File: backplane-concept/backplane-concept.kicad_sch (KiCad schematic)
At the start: 77 parts, among them IC1 ISO6760DWR, IC2 ISO6760DWR, J1 ECVT I/O, J11 1-967657-1, J12 POWER, J2 PCIE_8x_Labeled, J3 PCIE_8x_Labeled, J4 PCIE_8x_Labeled, J5 CONN_MINI, J6 CONN_MINI, J7 CONN_MINI, J8 CONN_MINI

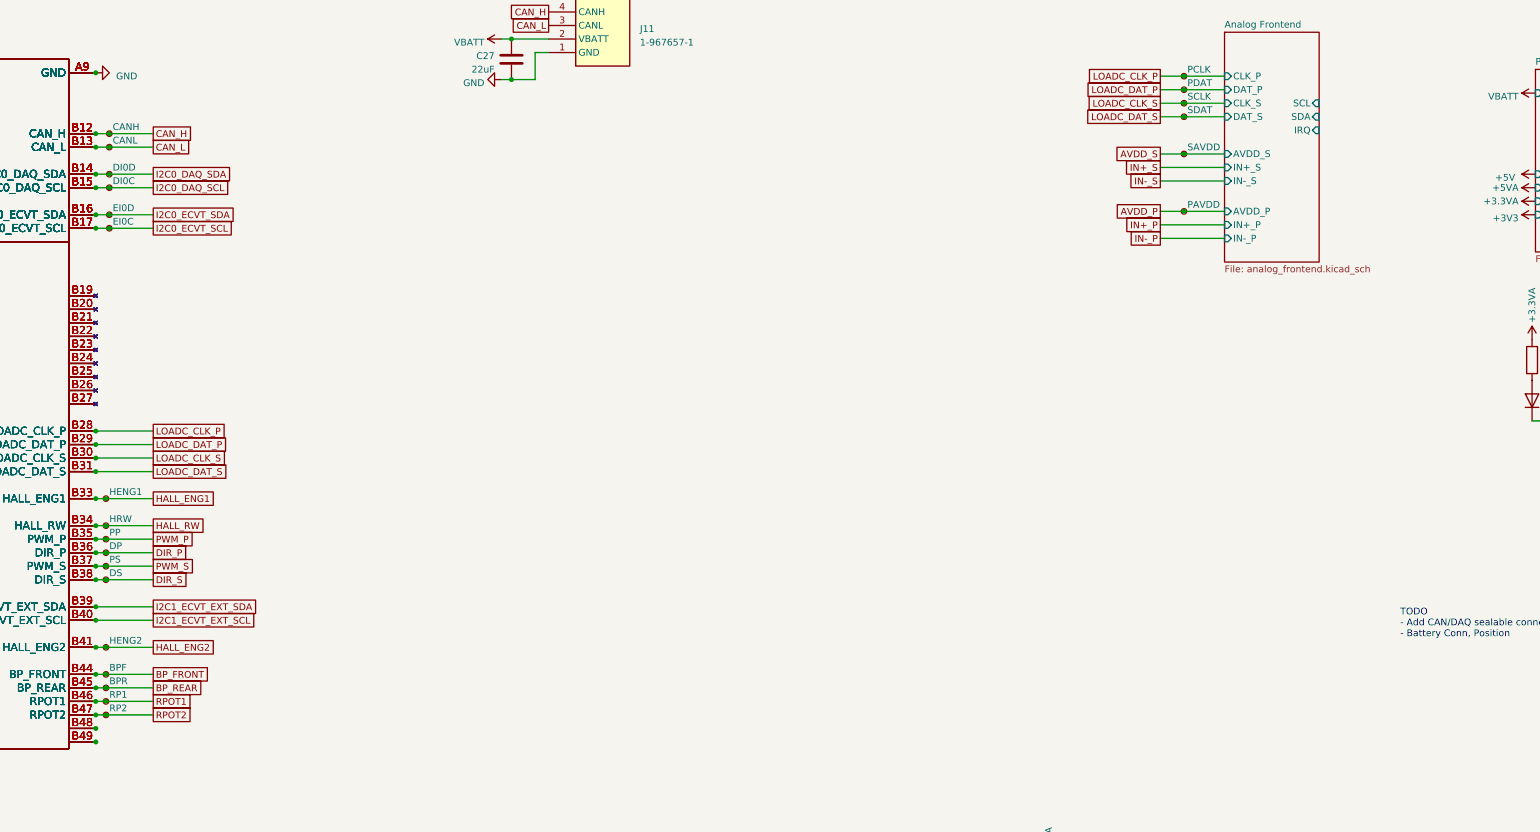
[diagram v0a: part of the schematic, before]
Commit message: Finish Routing
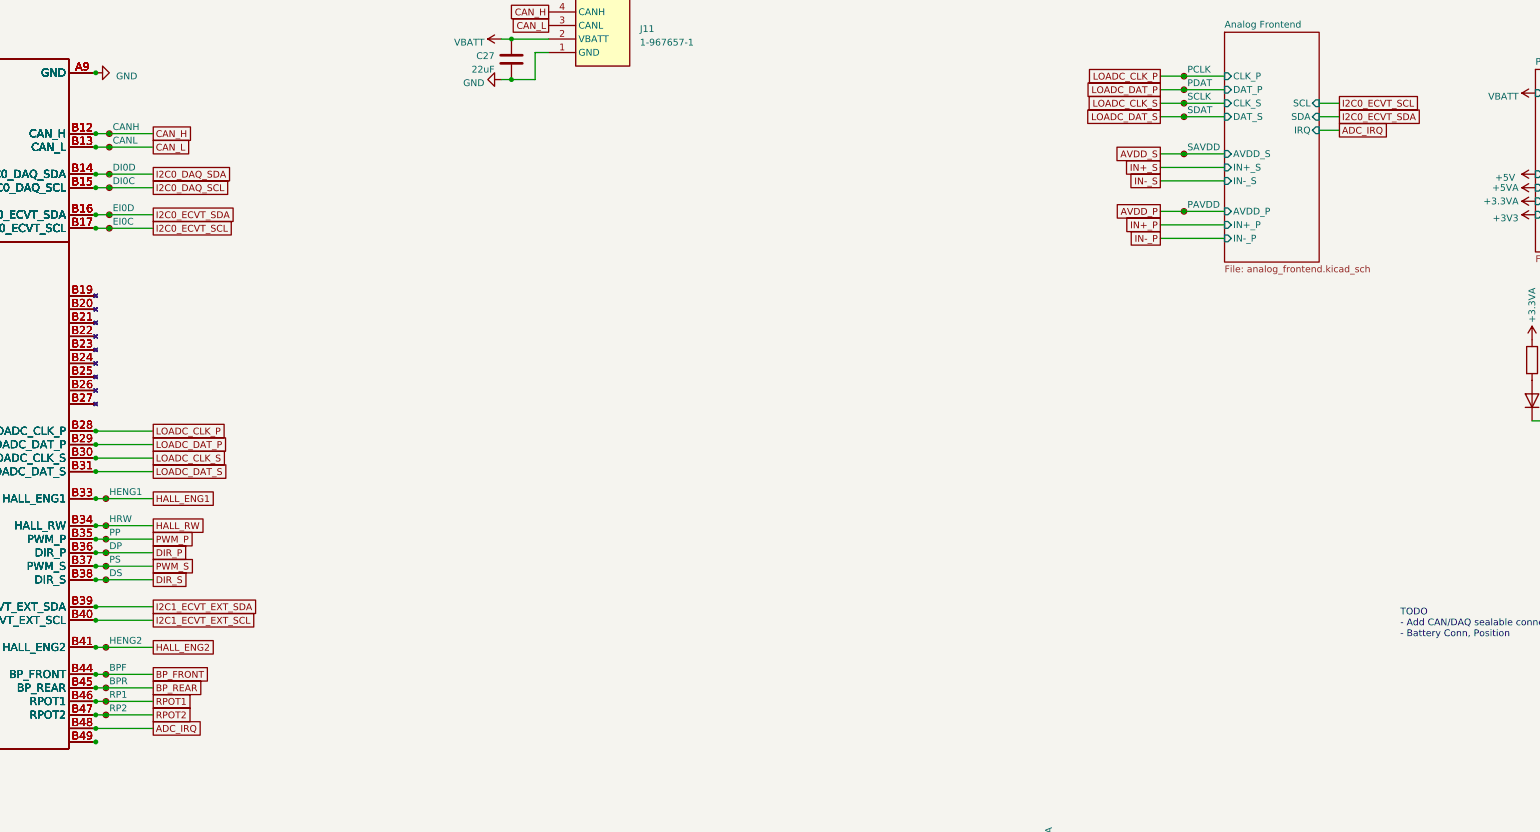
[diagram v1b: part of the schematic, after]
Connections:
- net ADC_IRQ: now reaches J2.B48, J3.B48, J4.B48
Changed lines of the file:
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@@
+    (stroke (width 0) (type default))
+  )
+  (wire (pts (xy 326.39 34.29) (xy 330.2 34.29))
     (stroke (width 0) (type default))
   )
@@
     (stroke (width 0) (type default))
   )
+  (wire (pts (xy 96.52 149.225) (xy 107.315 149.225))
+    (stroke (width 0) (type default))
+  )
   (wire (pts (xy 107.315 100.965) (xy 96.52 100.965))
     (stroke (width 0) (type default))
@@
     (stroke (width 0) (type default))
   )
+  (wire (pts (xy 326.39 36.83) (xy 330.2 36.83))
+    (stroke (width 0) (type default))
+  )
   (wire (pts (xy 36.195 121.285) (xy 38.1 121.285))
     (stroke (width 0) (type default))
@@
   )
   (wire (pts (xy 107.315 113.665) (xy 98.425 113.665))
+    (stroke (width 0) (type default))
+  )
+  (wire (pts (xy 326.39 31.75) (xy 330.2 31.75))
     (stroke (width 0) (type default))
   )
@@
     )
   )
+  (global_label "ADC_IRQ" (shape passive) (at 330.2 36.83 0) (fields_autoplaced)
+    (effects (font (size 1.27 1.27)) (justify left))
+    (property "Intersheetrefs" "${INTERSHEET_REFS}" (at 339.796 36.83 0)
+      (effects (font (size 1.27 1.27)) (justify left) hide)
+    )
+  )
   (global_label "I2C0_ECVT_SDA" (shape passive) (at 107.315 52.705 0) (fields_autoplaced)
     (effects (font (size 1.27 1.27)) (justify left))
@@
     (property "Intersheetrefs" "${INTERSHEET_REFS}" (at 289.0052 57.15 0)
       (effects (font (size 1.27 1.27)) (justify right) hide)
+    )
+  )
+  (global_label "I2C0_ECVT_SCL" (shape passive) (at 330.2 31.75 0) (fields_autoplaced)
+    (effects (font (size 1.27 1.27)) (justify left))
+    (property "Intersheetrefs" "${INTERSHEET_REFS}" (at 346.2063 31.75 0)
+      (effects (font (size 1.27 1.27)) (justify left) hide)
     )
   )
@@
     )
   )
+  (global_label "ADC_IRQ" (shape passive) (at 107.315 149.225 0) (fields_autoplaced)
+    (effects (font (size 1.27 1.27)) (justify left))
+    (property "Intersheetrefs" "${INTERSHEET_REFS}" (at 116.911 149.225 0)
+      (effects (font (size 1.27 1.27)) (justify left) hide)
+    )
+  )
+  (global_label "I2C0_ECVT_SDA" (shape passive) (at 330.2 34.29 0) (fields_autoplaced)
+    (effects (font (size 1.27 1.27)) (justify left))
+    (property "Intersheetrefs" "${INTERSHEET_REFS}" (at 346.2668 34.29 0)
+      (effects (font (size 1.27 1.27)) (justify left) hide)
+    )
+  )
